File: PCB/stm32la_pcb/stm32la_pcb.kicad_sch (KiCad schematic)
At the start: 18 parts, among them J1 Conn_01x04_Pin, J2 Conn_01x04_Pin, SW1 SW_SPDT, U1 STM32F103C8Tx, Y1 Crystal

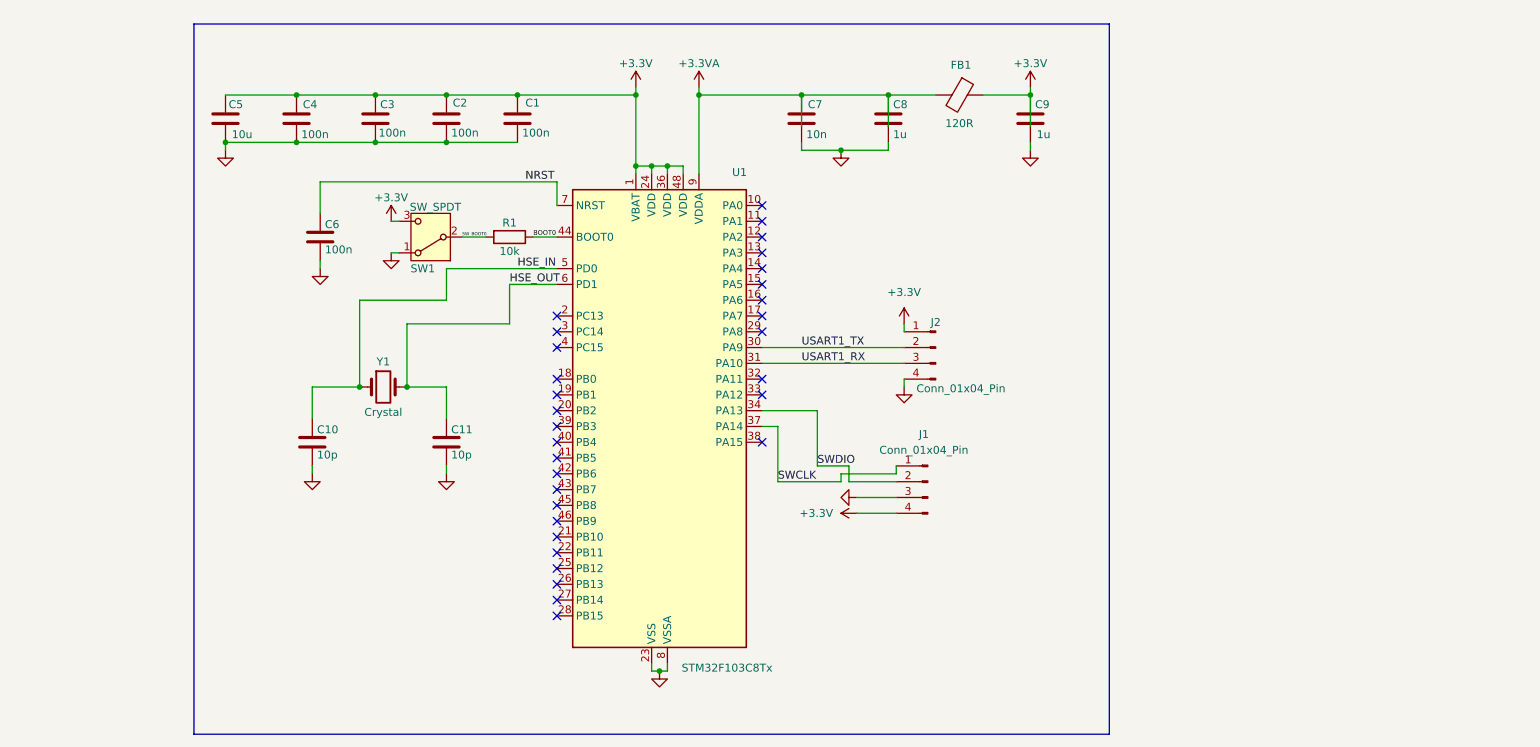
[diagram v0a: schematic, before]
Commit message: pcb
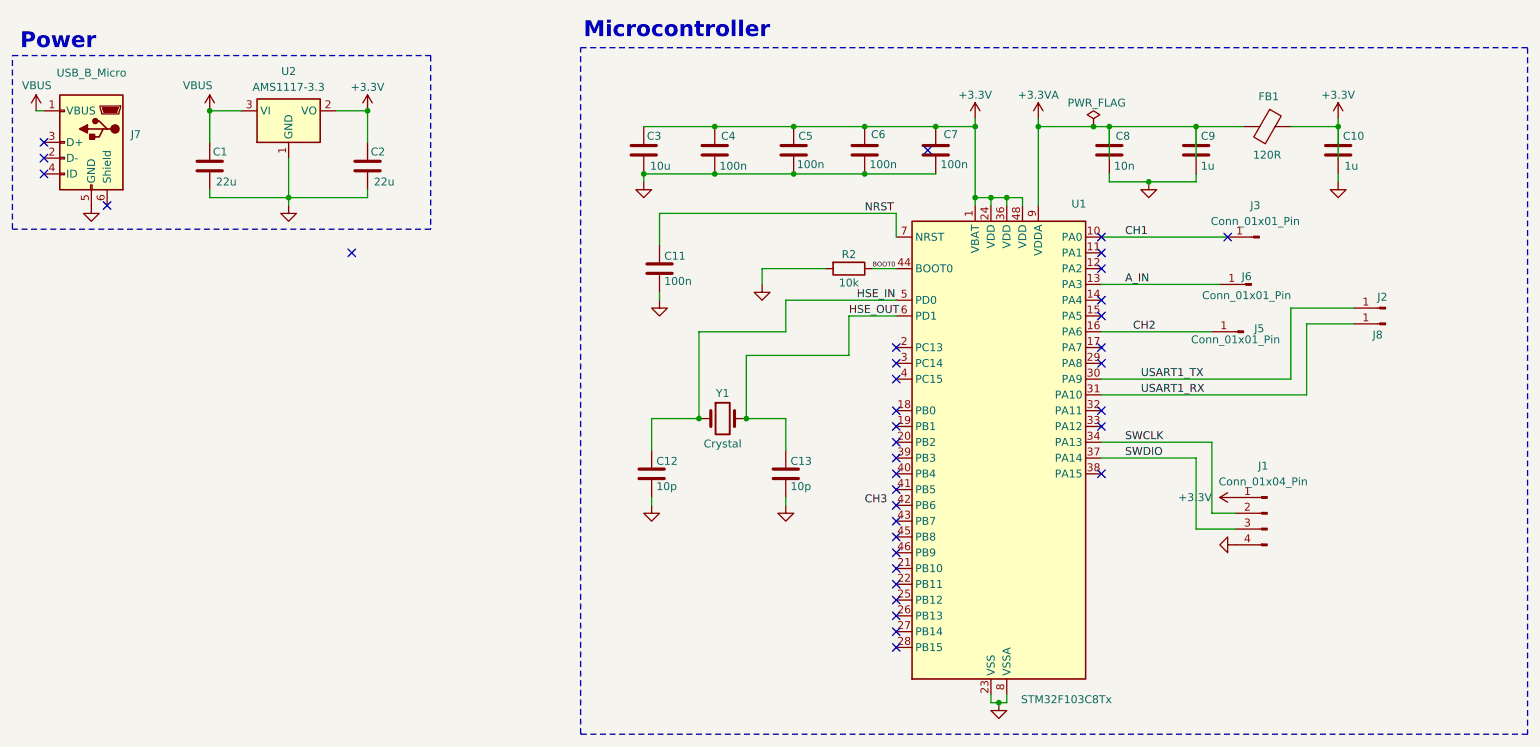
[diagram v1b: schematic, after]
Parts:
- removed J2: Conn_01x04_Pin, symbol Connector:Conn_01x04_Pin
- removed SW1: SW_SPDT, symbol Switch:SW_SPDT
- added C1, C2: 22u, Capacitor_THT:C_Disc_D3.0mm_W2.0mm_P2.50mm, symbol Device:C
- added J2, J3, J5, J6, J8: Conn_01x01_Pin, Connector_PinHeader_2.54mm:PinHeader_1x01_P2.54mm_Vertical, symbol Connector:Conn_01x01_Pin
- added J7: USB_B_Micro, Connector_USB:USB_Micro-B_Wuerth_629105150521, symbol Connector:USB_B_Micro
- added U2: AMS1117-3.3, Package_TO_SOT_SMD:SOT-223-3_TabPin2, symbol Regulator_Linear:AMS1117-3.3
- C10: renamed from C9; footprint (none) -> Capacitor_THT:C_Disc_D3.0mm_W2.0mm_P2.50mm
- C11: renamed from C6; footprint (none) -> Capacitor_THT:C_Disc_D3.0mm_W2.0mm_P2.50mm
- C12: renamed from C10; footprint (none) -> Capacitor_THT:C_Disc_D3.0mm_W1.6mm_P2.50mm
- C13: renamed from C11; footprint (none) -> Capacitor_THT:C_Disc_D3.0mm_W1.6mm_P2.50mm
- C3: renamed from C5; footprint (none) -> Capacitor_THT:C_Disc_D3.0mm_W2.0mm_P2.50mm
- C4: footprint (none) -> Capacitor_THT:C_Disc_D3.0mm_W2.0mm_P2.50mm
- C5: renamed from C3; footprint (none) -> Capacitor_THT:C_Disc_D3.0mm_W2.0mm_P2.50mm
- C6: renamed from C2; footprint (none) -> Capacitor_THT:C_Disc_D3.0mm_W2.0mm_P2.50mm
- C7: renamed from C1; footprint (none) -> Capacitor_THT:C_Disc_D3.0mm_W2.0mm_P2.50mm
- C8: renamed from C7; footprint (none) -> Capacitor_THT:C_Disc_D3.0mm_W1.6mm_P2.50mm
- C9: renamed from C8; footprint (none) -> Capacitor_THT:C_Disc_D3.0mm_W2.0mm_P2.50mm
- FB1: footprint (none) -> Inductor_THT:L_Axial_L5.0mm_D3.6mm_P10.00mm_Horizontal_Murata_BL01RN1A2A2
- J1: footprint (none) -> Connector_PinHeader_2.54mm:PinHeader_1x04_P2.54mm_Vertical
- R2: renamed from R1; footprint (none) -> Resistor_THT:R_Axial_DIN0204_L3.6mm_D1.6mm_P5.08mm_Horizontal
- Y1: footprint (none) -> HC-49_U-S16000000ABJB:XTAL_HC49P488W43L1150T466H350
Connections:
- net SW_BOOT0 is gone; now on net GND: R2.2
- net +3.3V: now also J1.1 (Pin_1), C2.1, U2.2 (VO); no longer J1.4 (Pin_4)
- net GND: now also J1.4 (Pin_4), C1.2, C2.2, J7.5 (GND), U2.1 (GND); no longer J1.3 (Pin_3)
- net SWCLK: now also J1.2 (Pin_2), U1.34 (PA13); no longer J1.1 (Pin_1), U1.37 (PA14)
- net SWDIO: now also J1.3 (Pin_3), U1.37 (PA14); no longer J1.2 (Pin_2), U1.34 (PA13)
- net USART1_RX: now also J8.1 (Pin_1)
- net USART1_TX: now also J2.1 (Pin_1)
- net CH1: now reaches U1.10 (PA0)
- net CH1: now also J3.1 (Pin_1)
- net A_IN: now reaches U1.13 (PA3)
- net A_IN: now also J6.1 (Pin_1)
- net CH2: now reaches U1.16 (PA6)
- net CH2: now also J5.1 (Pin_1)
- new net VBUS: C1.1, J7.1 (VBUS), U2.3 (VI)
- no-connect marks 31 -> 36
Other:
- note added: "Microcontroller"
- note added: "Power"
- title: (none) -> STM32 Logic Analyzer
- moved on the sheet: C10, C11, C12, C13, C3, C4, C5, C6, C7, C8, C9, FB1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
